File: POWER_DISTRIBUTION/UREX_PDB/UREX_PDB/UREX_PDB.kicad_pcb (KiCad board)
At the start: 4 copper layers, 90 x 60 mm, 128 parts, among them IC1 TCAN1044VDDFR, IC10 TPS22997RYZR, IC2 TPS1HB08BQPWPRQ1, IC3 TPS1HB08BQPWPRQ1, IC4 INA232AIDDFR, IC5 TCA6408ARGTR, IC8 TPS22997RYZR, IC9 TPS22997RYZR, J1 S2B-PH-SM4-TB_LF__SN_, J10 S2B-PH-SM4-TB_LF__SN_, J11 Conn_01x02, J33 Conn_01x02, J34 Conn_01x02, J36 Conn_01x02, J37 Conn_01x02, J4 S2B-PH-SM4-TB_LF__SN_, J5 S3B-PH-SM4-TB_LF__SN_, J6 S4B-PH-SM4-TB_LF__SN_, J7 S2B-PH-SM4-TB_LF__SN_, J8 S3B-PH-SM4-TB_LF__SN_, J9 S6B-PH-SM4-TB_LF__SN_, Q1 RSS070N05HZGTB, Q2 RSS070N05HZGTB, U1 ESP32-WROOM-32UE-R2, U4 PLM1117120QDCYRQ1, U5 XTPS552892RYQR, U7 USBLC6-2SC6

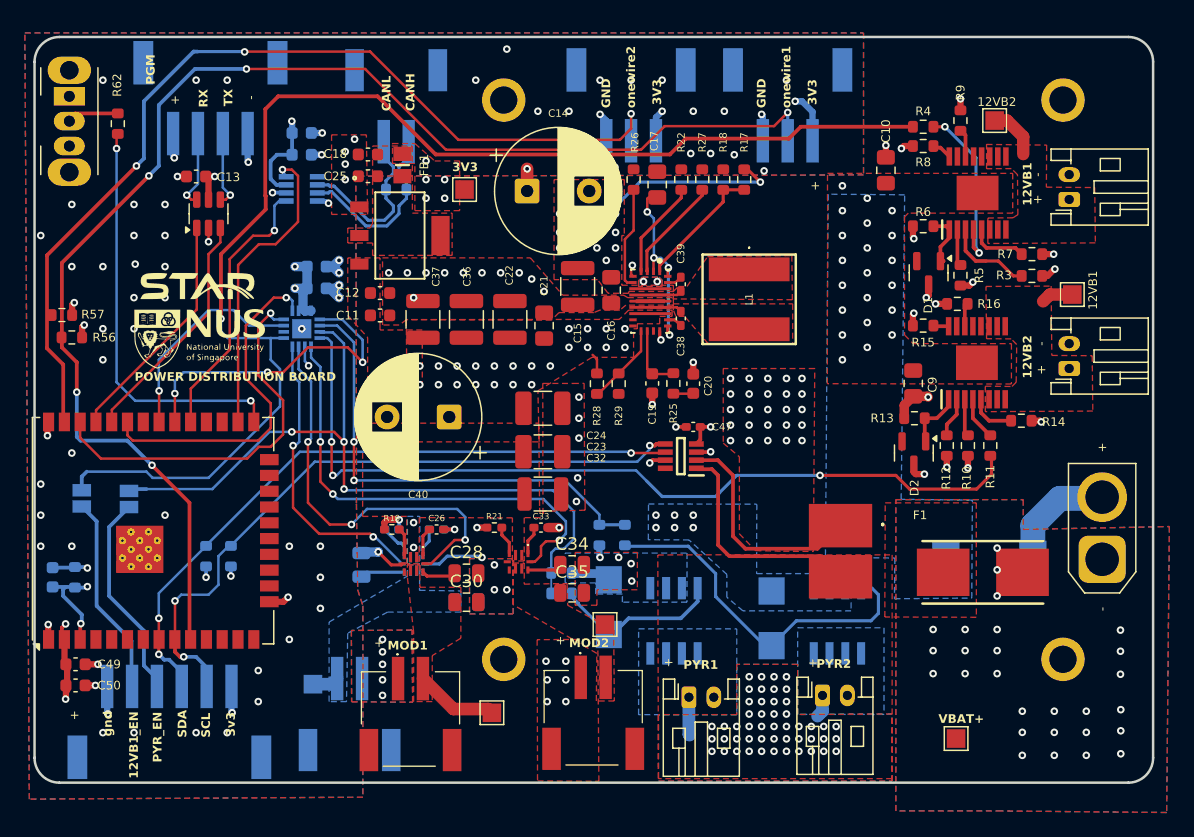
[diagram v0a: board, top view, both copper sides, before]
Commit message: V1 Full Fabrication(Freezed design)
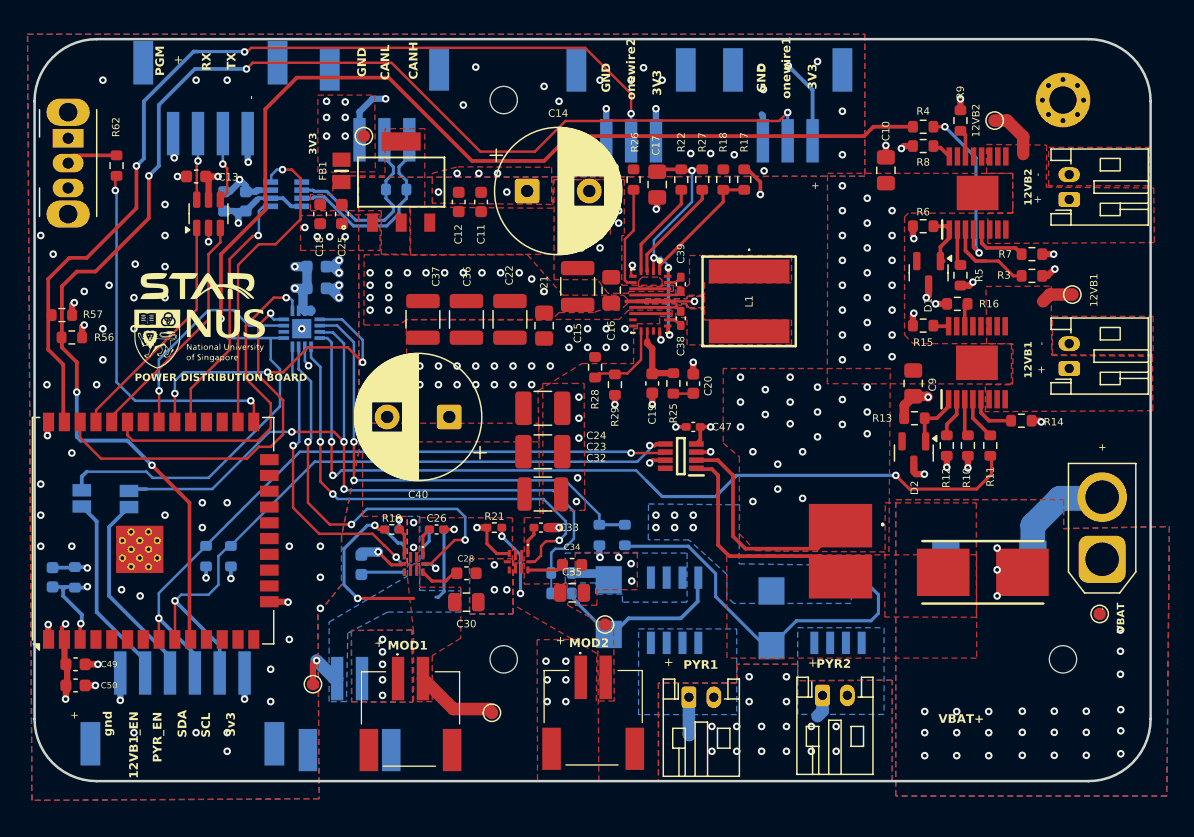
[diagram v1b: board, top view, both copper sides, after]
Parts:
- removed J1: S2B-PH-SM4-TB_LF__SN_, SamacSys_Parts:S2BPHSM4TBLFSN
- added J12: S3B-PH-SM4-TB_LF__SN_, SamacSys_Parts:S3BPHSM4TBLFSN, B.Cu at (110.2, 69.5)
- C20: value 18nF -> 22nF
- C28, C29, C34: value 1uF @50V -> 1nF; footprint Capacitor_SMD:C_0805_2012Metric -> Capacitor_SMD:C_0603_1608Metric
- H5, H7, H8: footprint MountingHole:MountingHole_2.2mm_M2_ISO7380_Pad -> MountingHole:MountingHole_2.2mm_M2_ISO7380
- H6: footprint MountingHole:MountingHole_2.2mm_M2_ISO7380_Pad -> MountingHole:MountingHole_2.2mm_M2_Pad_Via
- TP2, TP3, TP4, TP5, TP6, TP7: footprint TestPoint:TestPoint_Pad_1.5x1.5mm -> TestPoint:TestPoint_Pad_D1.0mm
- TP8: footprint TestPoint:TestPoint_Pad_1.5x1.5mm -> TestPoint:TestPoint_Pad_D1.0mm; moved to F.Cu
- moved TP2 15.3 mm to (167.7, 110.5)
- moved C11 12.2 mm to (117.9, 77.3), turned to 90 degrees
- moved C12 9.68 mm to (116.1, 77.3), turned to 90 degrees
- moved TP5 9.17 mm to (108.5, 72.0), turned to 180 degrees
- moved C52 7.29 mm to (97.2, 77.2), turned to -90 degrees
- moved C51 7.11 mm to (99.0, 77.2), turned to -90 degrees
- moved C18 6.15 mm to (105.0, 78.3), turned to -90 degrees
- moved FB1 4.92 mm to (106.7, 74.8)
- moved U4 4.30 mm to (111.5, 75.7), turned to 0 degrees
- moved C25 3.70 mm to (106.7, 78.3), turned to -90 degrees
- moved R62 3.38 mm to (88.6, 74.4)
- moved S1 3.38 mm to (84.7, 72.2)
- moved J9 1.51 mm to (93.9, 115.2)
- moved R28 1.33 mm to (127.1, 90.6)
- moved IC1 1.32 mm to (102.2, 76.7)
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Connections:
- C10 pad 2: VBAT+ -> VBAT_Fused_OUT
- C11 pad 1: +5V0 -> VBAT_Fused_OUT
- C12 pad 1: +5V0 -> VBAT_Fused_OUT
- C9 pad 2: VBAT+ -> VBAT_Fused_OUT
- IC2 pad 17: VBAT+ -> VBAT_Fused_OUT
- IC3 pad 17: VBAT+ -> VBAT_Fused_OUT
- J33 pad 1: VBAT_Fused -> VBAT_Fused_OUT
- J34 pad 1: VBAT_Fused -> VBAT_Fused_OUT
- R19 pad 1: +3V3 -> 5VDC_BUS1
- R20 pad 1: +3V3 -> 5VDC_BUS2
- R21 pad 1: +3V3 -> Net-(IC10-PG)
- R21 pad 2: Net-(IC10-PG) -> 5VDC_BUS3
- U4 pad 3: +5V0 -> VBAT_Fused_OUT
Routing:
- net 5VDC_BUS1: track 6.69 -> 19.8 mm, vias 0 -> 2
- net GND: track 76.8 -> 86.8 mm, vias 141 -> 159
- net 5VDC_BUS2: track 2.14 -> 10.1 mm, vias 0 -> 1
- net VBAT_Fused_OUT: track 33.0 -> 25.5 mm, vias 41 -> 77
- net /HighCurrentDCDC/DCDC_VCC: track 14.8 -> 21.5 mm
- net 5VDC_BUS3: track 0.07 -> 5.99 mm, vias 0 -> 2
- net VBAT_Fused: track 23.3 -> 18.4 mm, vias 49 -> 0
- net I2C2_SDL: track 53.4 -> 57.3 mm, vias 3 -> 2
- net +3V3: track 54.0 -> 50.6 mm
- net BOOT: track 33.1 -> 29.8 mm
- net VTX_EN_EXT: track 17.1 -> 14.5 mm
- net CAN_TX: track 22.1 -> 20.0 mm
- net Net-(IC10-PG): track 2.34 -> 4.23 mm, vias 0 -> 1
- net VTX_EN: track 105.7 -> 107.3 mm
- net +5V0: track 1.64 -> 0.00 mm
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- removed copper zone on In1.Cu, net VBAT+
- removed copper zone on B.Cu, net VBAT_Fused
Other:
- board size 90 x 60 mm -> 89.8 x 59.7 mm
- board text added: "VBAT"
